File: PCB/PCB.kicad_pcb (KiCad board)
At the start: 2 copper layers, 96 x 99.9 mm, 56 parts, among them J1 USB_C_Receptacle_USB2.0_14P, Q1 IRLML2060, SW1 SW_Push, SW2 SW_Push, U1 RP2040, U2 W25Q16JVSS, U4 XC6206P332MR, U5 USBLC6-2SC6, Y1 Crystal_GND24

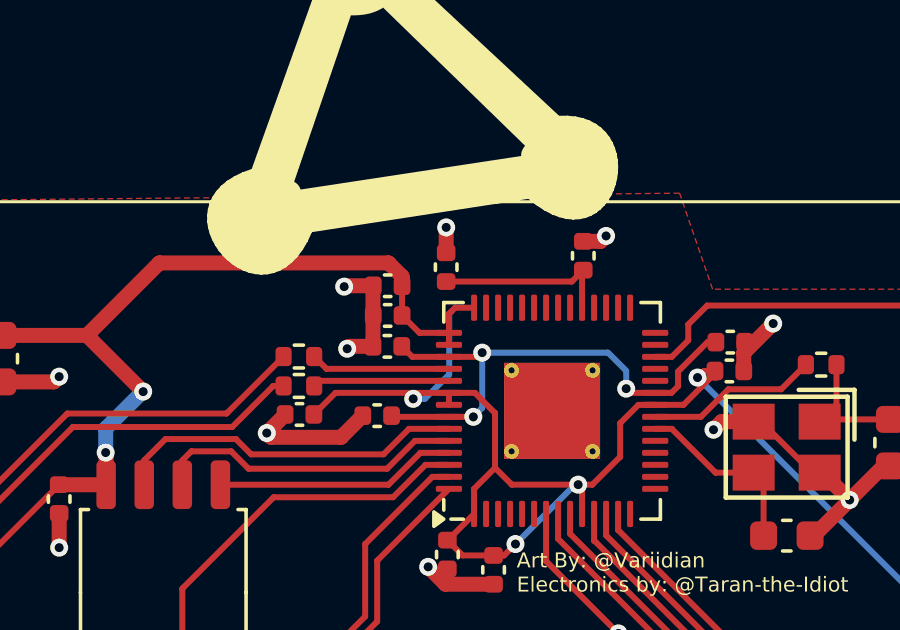
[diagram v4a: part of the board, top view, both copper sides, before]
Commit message: commit
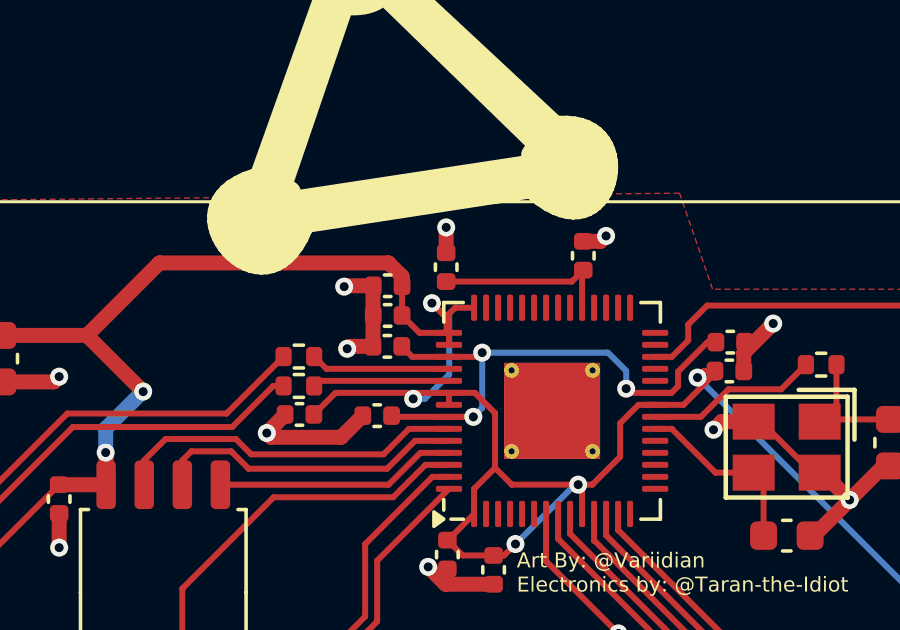
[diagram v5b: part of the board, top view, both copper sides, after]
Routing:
- net +3V3: track 180.0 -> 182.4 mm, vias 7 -> 8
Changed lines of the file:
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@@
+	)
+	(segment
+		(start 111.9925 59.3175)
+		(end 111.425 58.75)
+		(width 0.2)
+		(layer "F.Cu")
+		(net 1)
 	)
 	(segment
@@
 	)
 	(segment
+		(start 111.9925 59.74)
+		(end 111.9925 59.1075)
+		(width 0.2)
+		(layer "F.Cu")
+		(net 1)
+	)
+	(segment
 		(start 147.87 97.29)
 		(end 147.87 91.57)
@@
 	)
 	(segment
-		(start 111.9925 59.1075)
-		(end 112 59.1)
-		(width 0.2)
-		(layer "F.Cu")
-		(net 1)
-	)
-	(segment
 		(start 100.565 64.8025)
 		(end 99.0025 64.8025)
@@
 	)
 	(segment
+		(start 111.9125 59.66)
+		(end 111.9925 59.74)
+		(width 0.2)
+		(layer "F.Cu")
+		(net 1)
+	)
+	(segment
 		(start 100.565 63.745)
 		(end 100.55 63.73)
@@
 	)
 	(segment
-		(start 112.075 59.025)
-		(end 112 59.1)
-		(width 0.2)
-		(layer "F.Cu")
-		(net 1)
-	)
-	(segment
 		(start 96.925 59.65)
 		(end 97.1 59.825)
@@
 	)
 	(segment
-		(start 112.83 58.9025)
-		(end 112.1975 58.9025)
-		(width 0.2)
-		(layer "F.Cu")
-		(net 1)
-	)
-	(segment
 		(start 110.49 59.1)
 		(end 110.43 59.16)
@@
 	)
 	(segment
+		(start 111.9925 59.1075)
+		(end 112.1975 58.9025)
+		(width 0.2)
+		(layer "F.Cu")
+		(net 1)
+	)
+	(segment
 		(start 113.48 67.16)
 		(end 113.83 67.16)
@@
 	)
 	(segment
-		(start 112.1975 58.9025)
-		(end 112.075 59.025)
-		(width 0.2)
-		(layer "F.Cu")
-		(net 1)
-	)
-	(segment
 		(start 142.974 70.407)
 		(end 142.323 70.407)
@@
 	)
 	(segment
+		(start 111.9125 59.2375)
+		(end 111.9125 59.66)
+		(width 0.2)
+		(layer "F.Cu")
+		(net 1)
+	)
+	(segment
 		(start 111.9925 62.14)
 		(end 111.9925 61.74)
@@
 	)
 	(segment
-		(start 111.9925 59.74)
-		(end 111.9925 59.1075)
-		(width 0.2)
-		(layer "F.Cu")
-		(net 1)
-	)
-	(segment
 		(start 116.772 64.8)
 		(end 116.3 64.8)
@@
 	)
 	(segment
+		(start 112.1975 58.9025)
+		(end 112.83 58.9025)
+		(width 0.2)
+		(layer "F.Cu")
+		(net 1)
+	)
+	(segment
 		(start 119.81 62.14)
 		(end 120.86 61.09)
@@
 	)
 	(segment
+		(start 111.425 58.75)
+		(end 111.9125 59.2375)
+		(width 0.2)
+		(layer "F.Cu")
+		(net 1)
+	)
+	(segment
 		(start 146.9 73.9)
 		(end 143.407 70.407)
@@
 	)
 	(segment
+		(start 111.9925 59.74)
+		(end 111.9925 59.3175)
+		(width 0.2)
+		(layer "F.Cu")
+		(net 1)
+	)
+	(segment
 		(start 139.86 70.52)
 		(end 142.21 70.52)
@@
 		(net 1)
 	)
+	(via
+		(at 111.425 58.75)
+		(size 0.6)
+		(drill 0.3)
+		(layers "F.Cu" "B.Cu")
+		(net 1)
+	)

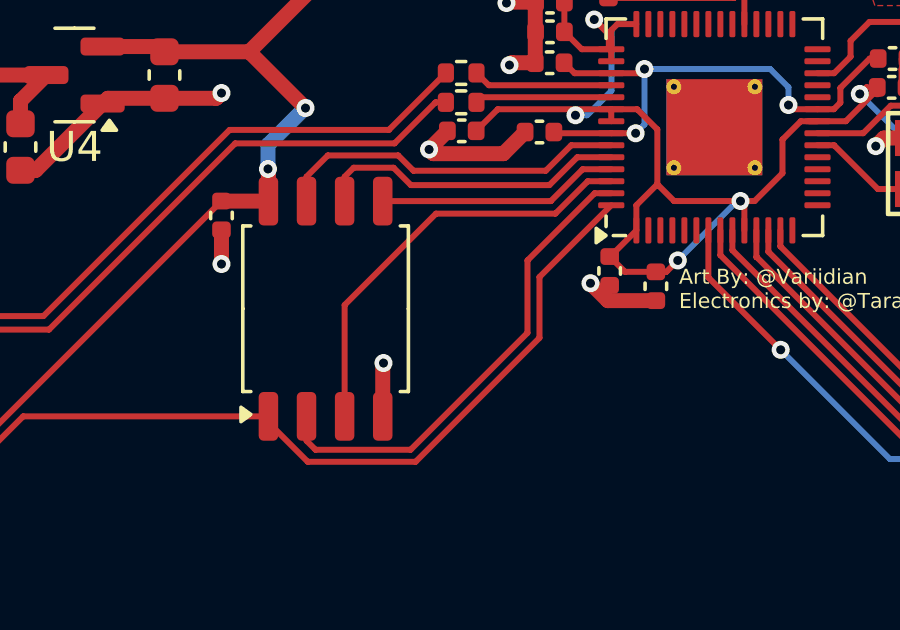
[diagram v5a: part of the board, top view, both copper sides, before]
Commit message: banana
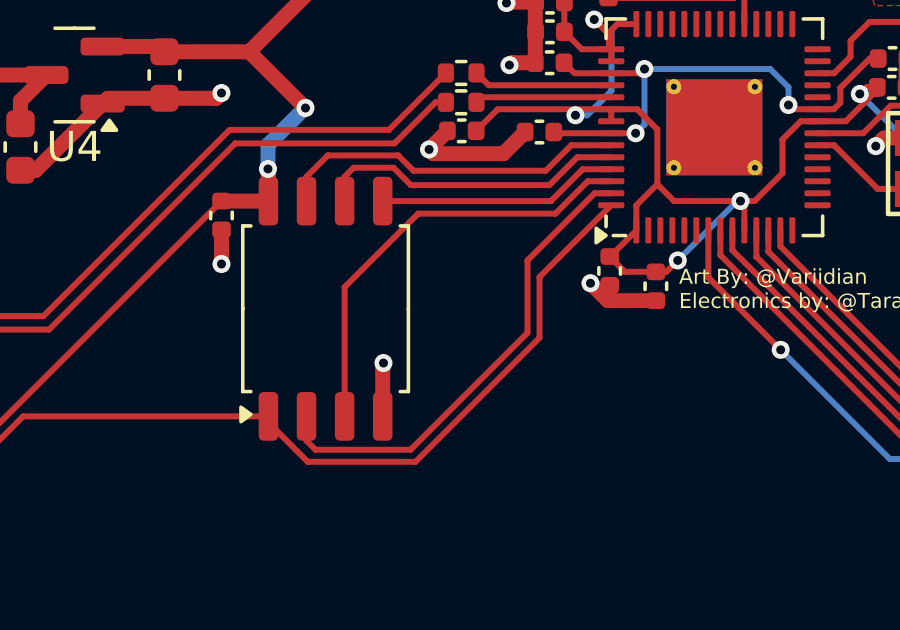
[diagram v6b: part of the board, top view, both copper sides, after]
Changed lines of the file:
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@@
 	)
 	(segment
-		(start 103.105 68.265)
-		(end 103.105 71.9775)
+		(start 110.13 65.22)
+		(end 105.555 65.22)
 		(width 0.2)
 		(layer "F.Cu")
@@
 	)
 	(segment
-		(start 111.9925 64.14)
-		(end 111.21 64.14)
-		(width 0.2)
-		(layer "F.Cu")
-		(net 48)
-	)
-	(segment
-		(start 106.15 65.22)
-		(end 103.105 68.265)
+		(start 103.105 67.67)
+		(end 103.105 71.9775)
 		(width 0.2)
 		(layer "F.Cu")
@@
 	)
 	(segment
-		(start 110.13 65.22)
-		(end 106.15 65.22)
+		(start 105.555 65.22)
+		(end 103.105 67.67)
 		(width 0.2)
 		(layer "F.Cu")
+		(net 48)
+	)
+	(segment
+		(start 111.9925 64.14)
+		(end 111.21 64.14)
+		(width 0.2)
+		(layer "F.Cu")
